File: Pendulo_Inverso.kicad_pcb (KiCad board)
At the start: 2 copper layers, 55.9 x 63.5 mm, 10 parts, among them IC2 TB6612FNG, U1 LM7805_TO220, U2 ESP32-DEVKITC, U4 MPU-6050-A

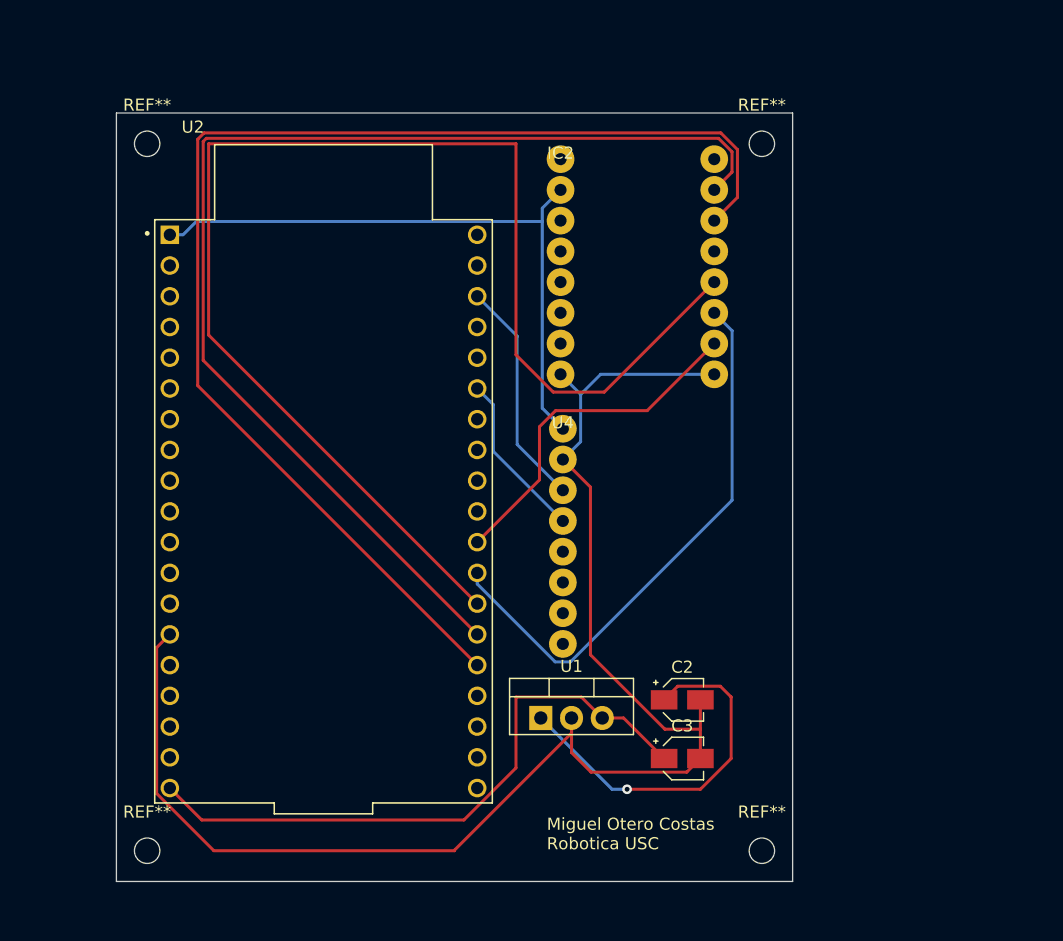
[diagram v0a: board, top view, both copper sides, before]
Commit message: modified:   Pendulo_Inverso.dsn 	modified:   Pendulo_Inverso.kicad_pcb 	modified:   Pendulo_Inverso.kicad_prl 	modified:   Pendulo_Inverso.kicad_sch 	modified:   Pendulo_Inverso.rules 	modified:   Pendulo_Inverso.ses 	modified:   fp-info-cache
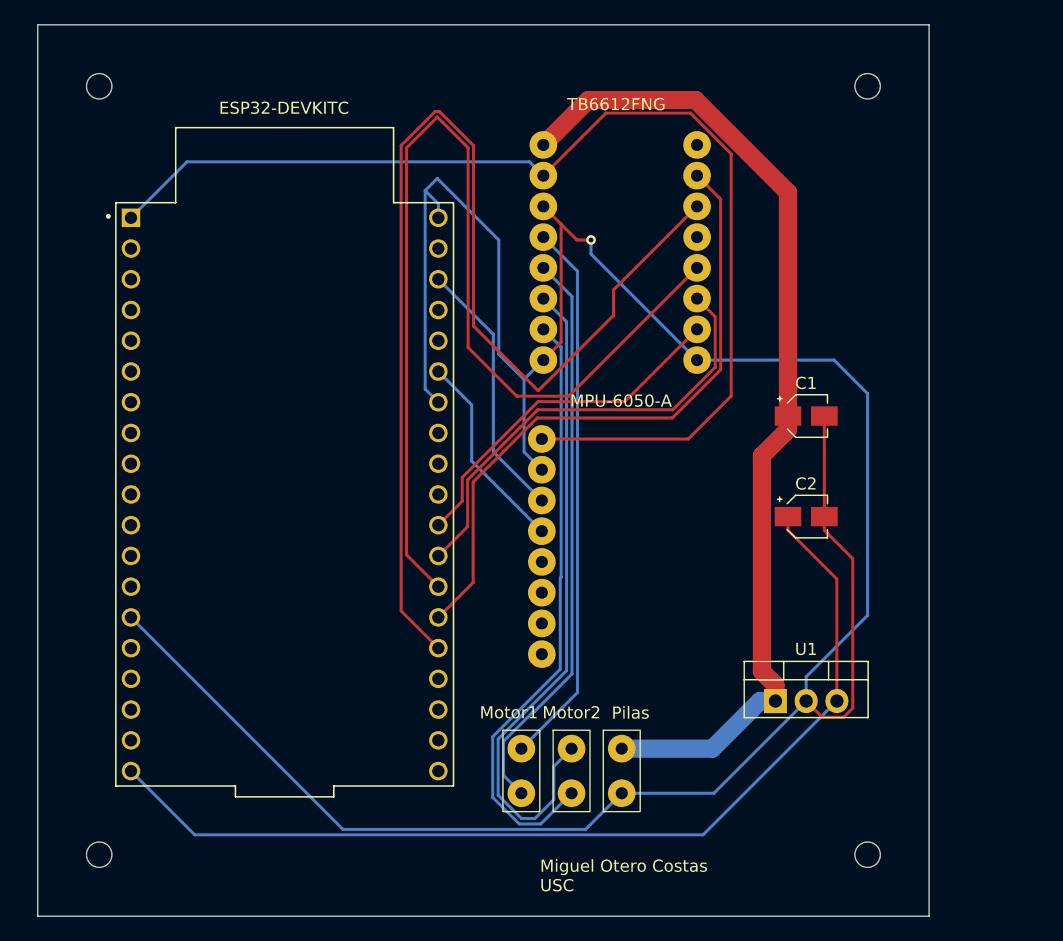
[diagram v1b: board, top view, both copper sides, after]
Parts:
- removed C3: 0.1uF, Capacitor_SMD:CP_Elec_3x5.3
- removed IC2: TB6612FNG, Mi_Libreria2:TB6612FNG
- removed the REF** at (116.8, 78.7)
- removed the REF** at (167.6, 137.2)
- removed the REF** at (116.8, 137.2)
- removed U2: ESP32-DEVKITC, Mi_Libreria2:MODULE_ESP32-DEVKITC
- removed U4: MPU-6050-A, Mi_Libreria2:MPU6050
- added C1: 0.33uF, Capacitor_SMD:CP_Elec_3x5.3, F.Cu at (171.3, 101.2)
- added ESP32-DEVKITC: ESP32-DEVKITC, Mi_Libreria2:MODULE_ESP32-DEVKITC, F.Cu at (128.2, 107.7)
- added MPU-6050-A: MPU-6050-A, Mi_Libreria2:MPU6050, F.Cu at (149.5, 103.1)
- added Motor1: ~, Mi_Libreria2:Conector_doble, F.Cu at (147.8, 128.7)
- added Motor2: ~, Mi_Libreria2:Conector_doble, F.Cu at (151.9, 128.7)
- added Pilas: ~, Mi_Libreria2:Conector_doble, F.Cu at (156.1, 128.7)
- added REF**: MountingHole_2.1mm, MountingHole:MountingHole_2.1mm, F.Cu at (112.9, 137.5)
- added REF**: MountingHole_2.1mm, MountingHole:MountingHole_2.1mm, F.Cu at (112.9, 74.0)
- added REF**: MountingHole_2.1mm, MountingHole:MountingHole_2.1mm, F.Cu at (176.4, 137.5)
- added TB6612FNG: TB6612FNG, Mi_Libreria2:TB6612FNG, F.Cu at (149.6, 78.8)
- C2: value 0.33uF -> 0.1uF
- moved U1 19.4 mm to (168.8, 124.8)
- moved C2 18.3 mm to (171.3, 109.5)
- moved REF** 9.95 mm to (176.4, 74.0)
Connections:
- C2 pad 1: Net-(U1-VI) -> Net-(U1-VO)
- U1 pad 1: Net-(U1-VI) -> Net-(IC2-VM1)
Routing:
- net GND: track 123.9 -> 222.5 mm, vias 0 -> 1
- net Net-(IC2-VM1): track 0.00 -> 82.6 mm
- net BO1: track 0.00 -> 55.0 mm
- net BO2: track 0.00 -> 50.1 mm
- net AO2: track 0.00 -> 47.4 mm
- net AO1: track 0.00 -> 45.4 mm
- net AIN1: track 98.1 -> 53.5 mm
- net VCC: track 52.3 -> 92.7 mm
- net Net-(U1-VI): track 30.7 -> 0.00 mm, vias 1 -> 0
- net Net-(U1-VO): track 51.7 -> 82.0 mm
- net BIN1: track 111.5 -> 86.0 mm
- net AIN2: track 105.1 -> 94.3 mm
- net BIN2: track 46.3 -> 37.9 mm
- net Net-(U2-IO22): track 19.0 -> 21.8 mm
- net Net-(U2-IO21): track 13.9 -> 16.7 mm
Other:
- board size 55.9 x 63.5 mm -> 73.7 x 73.7 mm
- board text added: "Miguel Otero Costas USC"
- board text removed: "Miguel Otero Costas Robotica USC"

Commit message: new file:   Pendulo_Inverso-backups/Pendulo_Inverso-2024-04-04_134628.zip 	modified:   Pendulo_Inverso.kicad_pcb 	modified:   Pendulo_Inverso.kicad_prl 	modified:   Pendulo_Inverso.kicad_pro 	modified:   Pendulo_Inverso.kicad_sch 	modified:   fp-info-cache
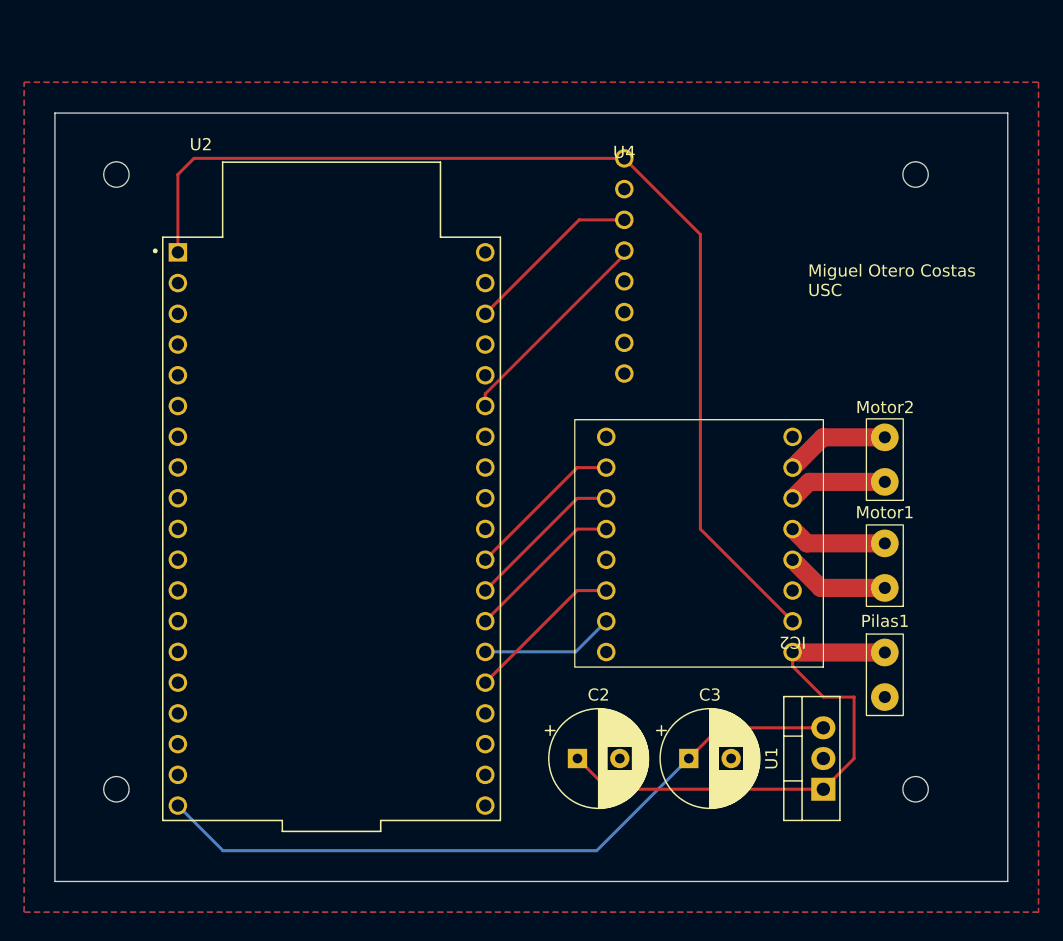
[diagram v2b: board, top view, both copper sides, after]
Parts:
- removed C1: 0.33uF, Capacitor_SMD:CP_Elec_3x5.3
- removed ESP32-DEVKITC: ESP32-DEVKITC, Mi_Libreria2:MODULE_ESP32-DEVKITC
- removed MPU-6050-A: MPU-6050-A, Mi_Libreria2:MPU6050
- removed Pilas: ~, Mi_Libreria2:Conector_doble
- removed the REF** at (112.9, 137.5)
- removed the REF** at (112.9, 74.0)
- removed the REF** at (176.4, 137.5)
- removed the REF** at (176.4, 74.0)
- removed TB6612FNG: TB6612FNG, Mi_Libreria2:TB6612FNG
- added C3: 0.1uF, Capacitor_THT:CP_Radial_D8.0mm_P3.50mm, F.Cu at (161.6, 129.5)
- added IC2: TB6612FNG, Mi_Libreria2:TB6612FNG, F.Cu at (170.2, 119.4)
- added Pilas1: ~, Mi_Libreria2:Conector_doble, F.Cu at (177.8, 120.8)
- added REF**: MountingHole_2.1mm, MountingHole:MountingHole_2.1mm, F.Cu at (114.3, 132.1)
- added REF**: MountingHole_2.1mm, MountingHole:MountingHole_2.1mm, F.Cu at (180.3, 81.3)
- added REF**: MountingHole_2.1mm, MountingHole:MountingHole_2.1mm, F.Cu at (180.3, 132.1)
- added REF**: MountingHole_2.1mm, MountingHole:MountingHole_2.1mm, F.Cu at (114.3, 81.3)
- added U2: ESP32-DEVKITC, Mi_Libreria2:MODULE_ESP32-DEVKITC, F.Cu at (132.1, 110.6)
- added U4: MPU-6050-A, Mi_Libreria2:MPU6050, F.Cu at (156.3, 79.9)
- C2: value 0.1uF -> 0.33uF; footprint Capacitor_SMD:CP_Elec_3x5.3 -> Capacitor_THT:CP_Radial_D8.0mm_P3.50mm
- moved Motor2 34.0 mm to (177.8, 106.7), turned to 180 degrees
- moved Motor1 32.8 mm to (177.8, 115.4), turned to 180 degrees
- moved C2 27.5 mm to (152.4, 129.5)
- moved U1 8.30 mm to (172.7, 132.1), turned to 90 degrees
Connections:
- C2 pad 1: Net-(U1-VO) -> Net-(IC2-VM1)
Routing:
- net GND: track 222.5 -> 0.00 mm, vias 1 -> 0
- net AIN2: track 94.3 -> 13.2 mm
- net BIN1: track 86.0 -> 13.2 mm
- net BO1: track 55.0 -> 8.18 mm
- net AIN1: track 53.5 -> 11.0 mm
- net BO2: track 50.1 -> 8.66 mm
- net AO2: track 47.4 -> 8.11 mm
- net Net-(IC2-VM1): track 82.6 -> 45.0 mm
- net AO1: track 45.4 -> 8.58 mm
- net BIN2: track 37.9 -> 13.2 mm
- net Net-(U1-VO): track 82.0 -> 59.1 mm
- net PWMB: track 29.2 -> 13.2 mm
- net Net-(U2-IO22): track 21.8 -> 14.7 mm
- net VCC: track 92.7 -> 87.9 mm
- net Net-(U2-IO21): track 16.7 -> 17.6 mm
- added copper zone on B.Cu, net GND
- added copper zone on F.Cu, net GND
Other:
- board size 73.7 x 73.7 mm -> 78.7 x 63.5 mm
